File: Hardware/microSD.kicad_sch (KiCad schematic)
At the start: 6 parts, among them J3 Micro_SD_Card_Det, Q1 PMOS

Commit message: update
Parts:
- Q1: MPN (none) -> PNM723T201E0
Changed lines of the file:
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@@
+			)
+		)
+		(property "MPN" " PNM723T201E0"
+			(at 84.836 75.438 0)
+			(effects
+				(font
+					(size 1.27 1.27)
+				)
+				(hide yes)
 			)
 		)

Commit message: changes post 3rd review
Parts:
- Q1: footprint Package_TO_SOT_SMD:SOT-723 -> Package_TO_SOT_SMD:SOT-23; MPN PNM723T201E0 -> DMP3099L
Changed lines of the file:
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@@
 			)
 		)
-		(property "Footprint" "Package_TO_SOT_SMD:SOT-723"
+		(property "Footprint" "Package_TO_SOT_SMD:SOT-23"
 			(at 79.756 77.978 0)
 			(effects
@@
 			)
 		)
-		(property "MPN" " PNM723T201E0"
+		(property "MPN" " DMP3099L"
 			(at 84.836 75.438 0)
 			(effects

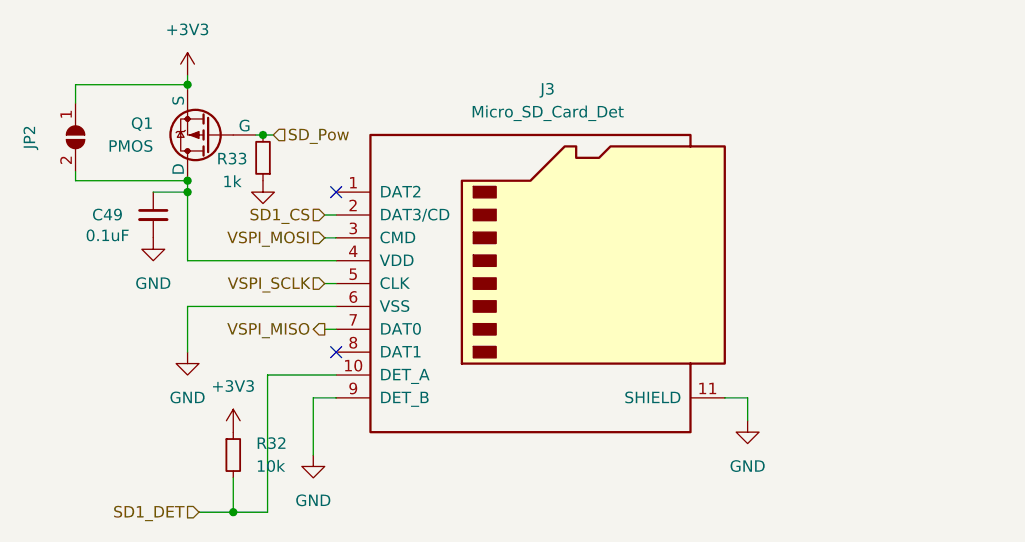
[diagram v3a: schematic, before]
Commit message: post Andrei review, new SD
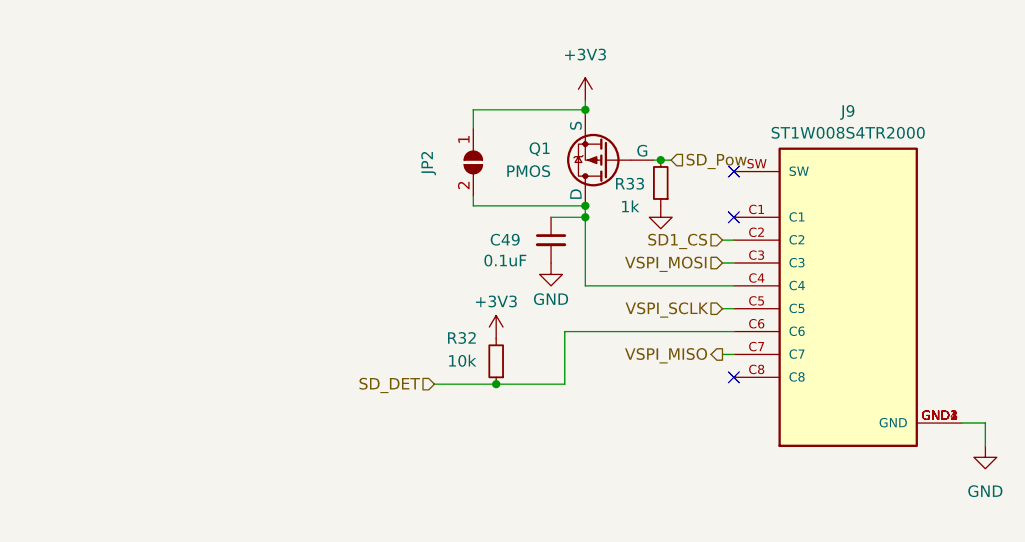
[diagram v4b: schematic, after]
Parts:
- removed J3: Micro_SD_Card_Det, Connector_Card:microSD_HC_Hirose_DM3AT-SF-PEJM5, symbol Connector:Micro_SD_Card_Det
- added J9: ST1W008S4TR2000, iclr:JAE_ST1W008S4TR2000, symbol iclr:ST1W008S4TR2000
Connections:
- net SD1_DET is gone; now on net +3V3: R32.2
- net +3V3: no longer R32.1
- net GND: now also J9.GND1 (GND), J9.GND2 (GND), J9.GND3 (GND), J9.GND4 (GND)
- net SD1_CS: now also J9.C2
- net VSPI_MISO: now also J9.C7
- net VSPI_MOSI: now also J9.C3
- net VSPI_SCLK: now also J9.C5
- net at C49.1, JP2.2 (B), Q1.1 (D): now also J9.C4
- new net SD_DET: J9.C6, R32.1
- no-connect marks 2 -> 3
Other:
- moved on the sheet: C49, JP2, Q1, R33
